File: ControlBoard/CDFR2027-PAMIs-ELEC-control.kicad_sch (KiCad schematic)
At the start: 14 parts

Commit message: (feat): bom
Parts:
- C1, C3: LCSC (none) -> C1591
- C2: LCSC (none) -> C59461
- ESP32-S3-WROOM1: LCSC (none) -> C3013946
- R1: LCSC (none) -> C22548
- R2, R24, R25: LCSC (none) -> C84376
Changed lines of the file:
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@@
+			)
+		)
+		(property "LCSC" "C1591"
+			(at 113.03 46.99 90)
+			(hide yes)
+			(show_name no)
+			(do_not_autoplace no)
+			(effects
+				(font
+					(size 1.27 1.27)
+				)
 			)
 		)
@@
 			)
 		)
+		(property "LCSC" "C22548"
+			(at 125.73 59.69 90)
+			(hide yes)
+			(show_name no)
+			(do_not_autoplace no)
+			(effects
+				(font
+					(size 1.27 1.27)
+				)
+			)
+		)
 		(pin "1"
 		)
@@
 			)
 		)
+		(property "LCSC" "C1591"
+			(at 143.51 48.26 90)
+			(hide yes)
+			(show_name no)
+			(do_not_autoplace no)
+			(effects
+				(font
+					(size 1.27 1.27)
+				)
+			)
+		)
 		(pin "2"
 		)
@@
 		(property "Description" "Resistor"
 			(at 176.53 104.14 0)
+			(hide yes)
+			(show_name no)
+			(do_not_autoplace no)
+			(effects
+				(font
+					(size 1.27 1.27)
+				)
+			)
+		)
+		(property "LCSC" "C84376"
+			(at 176.53 104.14 90)
 			(hide yes)
 			(show_name no)
@@
 			)
 		)
+		(property "LCSC" "C84376"
+			(at 176.53 106.68 90)
+			(hide yes)
+			(show_name no)
+			(do_not_autoplace no)
+			(effects
+				(font
+					(size 1.27 1.27)
+				)
+			)
+		)
 		(pin "1"
 		)
@@
 			)
 		)
+		(property "LCSC" "C84376"
+			(at 143.51 59.69 90)
+			(hide yes)
+			(show_name no)
+			(do_not_autoplace no)
+			(effects
+				(font
+					(size 1.27 1.27)
+				)
+			)
+		)
 		(pin "2"
 		)
@@
 			)
 		)
+		(property "LCSC" "C59461"
+			(at 143.51 36.83 90)
+			(hide yes)
+			(show_name no)
+			(do_not_autoplace no)
+			(effects
+				(font
+					(size 1.27 1.27)
+				)
+			)
+		)
 		(pin "2"
 		)
@@
 			(at 153.67 88.9 0)
 			(hide yes)
+			(show_name no)
+			(do_not_autoplace no)
+			(effects
+				(font
+					(size 1.27 1.27)
+				)
+			)
+		)
+		(property "LCSC" "C3013946"
+			(at 153.67 88.9 0)
+			(hide yes)

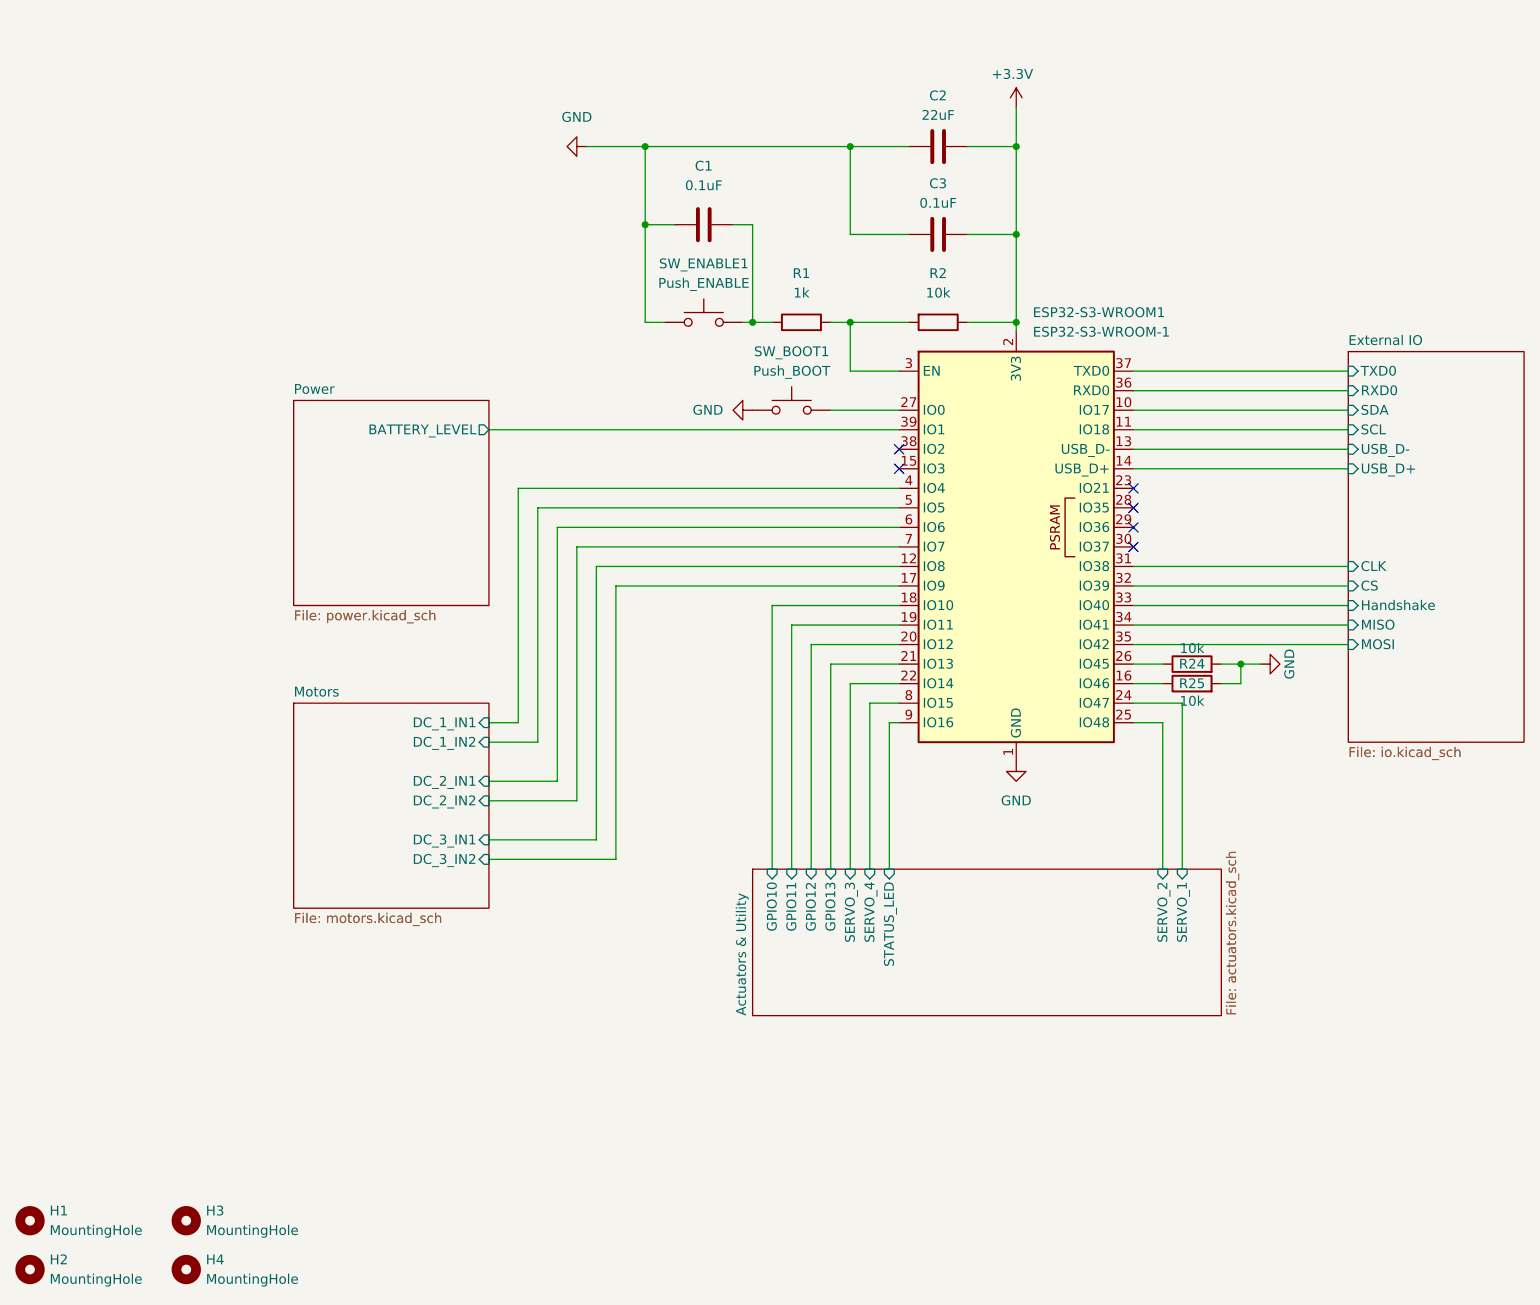
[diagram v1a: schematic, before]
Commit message: Updates to schematic by Ludo <3
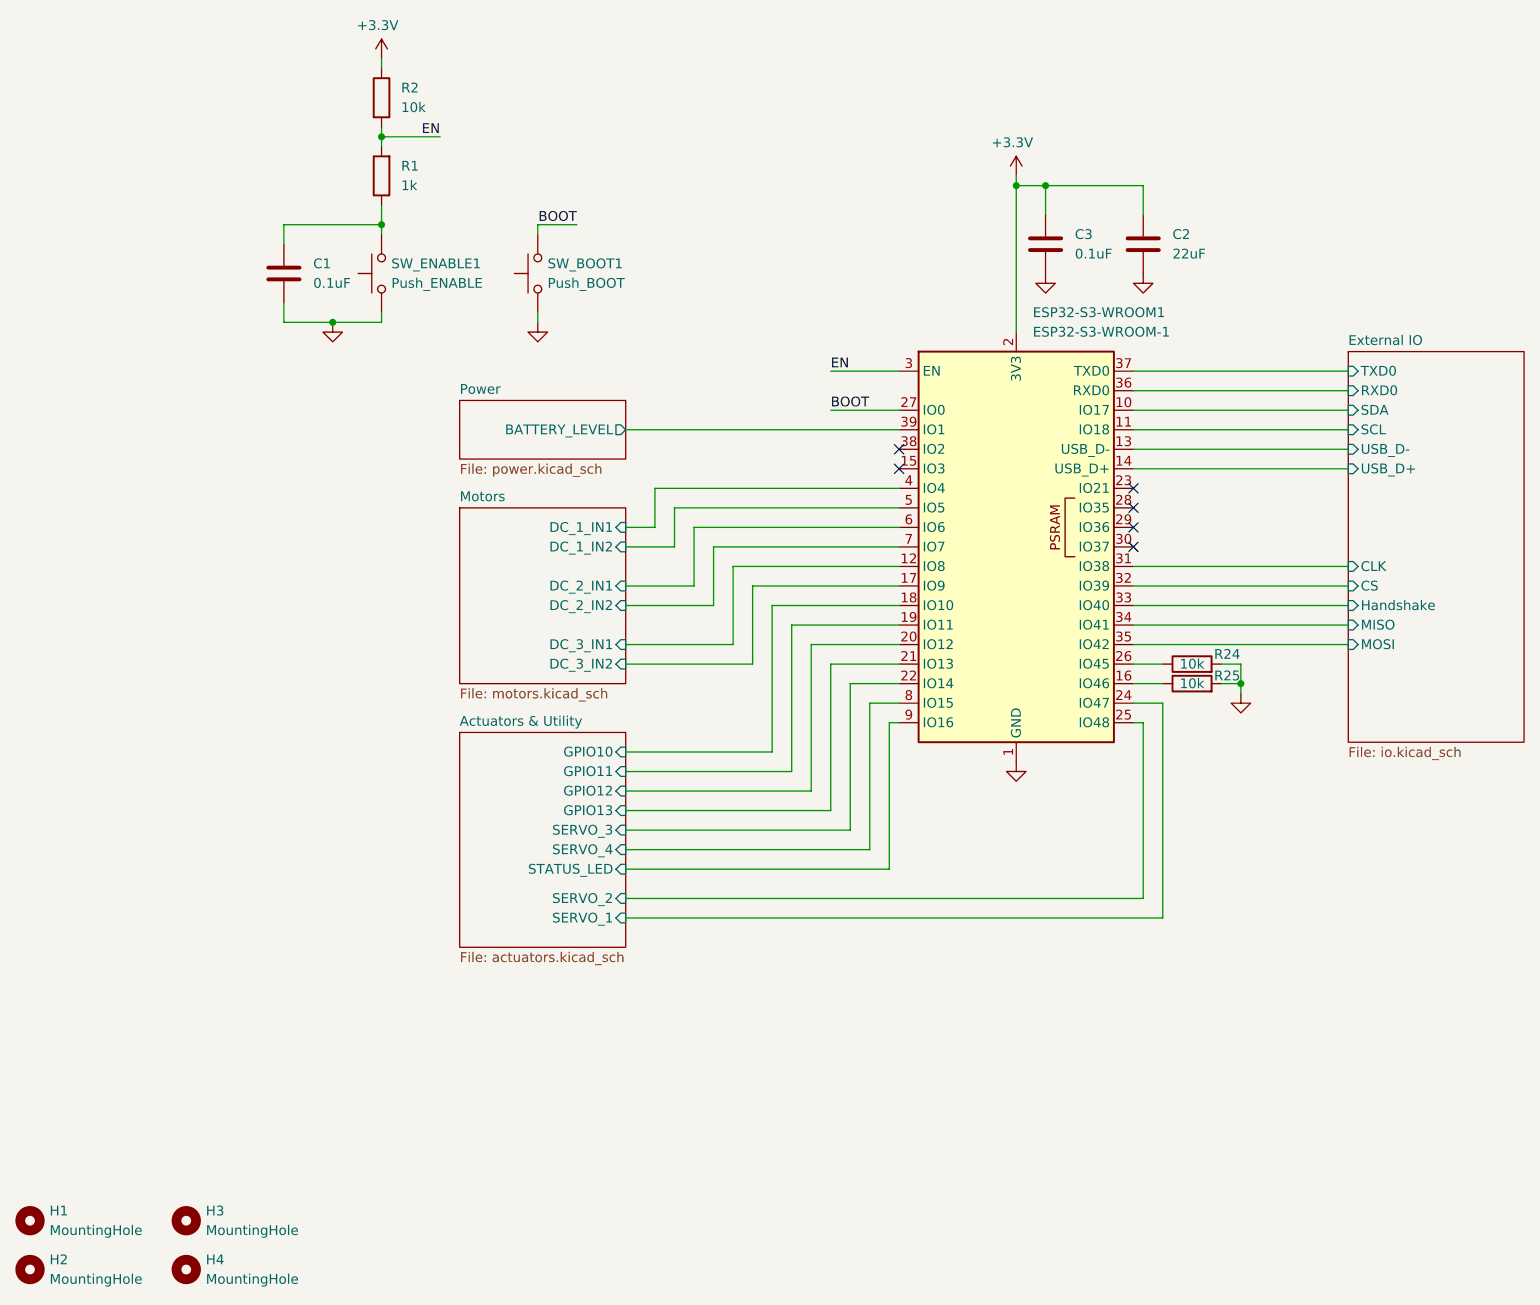
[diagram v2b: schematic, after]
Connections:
- net EN: now reaches ESP32-S3-WROOM1.3 (EN), R1.2, R2.2
- net BOOT: now reaches ESP32-S3-WROOM1.27 (IO0), SW_BOOT1.2
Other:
- moved on the sheet: C3
